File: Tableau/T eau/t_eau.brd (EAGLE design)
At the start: 70 x 60 mm, 24 parts

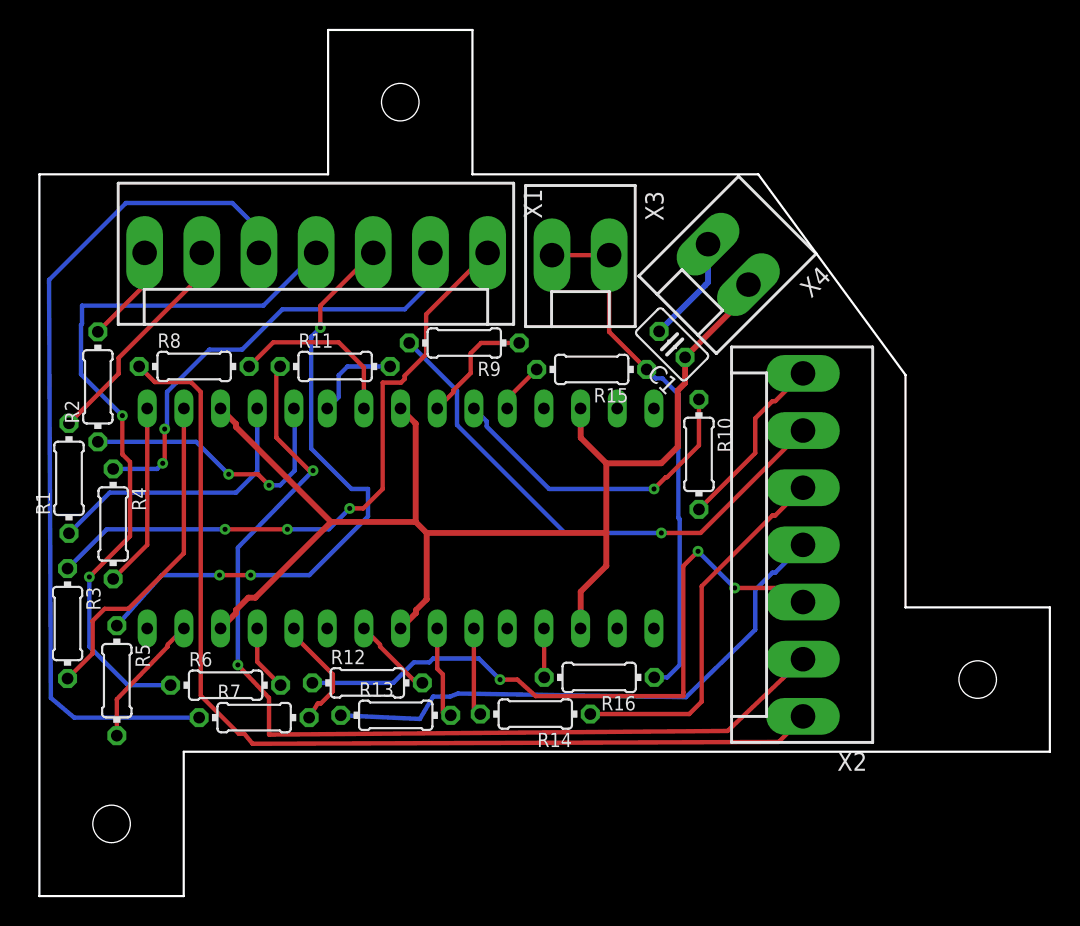
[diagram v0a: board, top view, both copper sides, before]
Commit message: no message
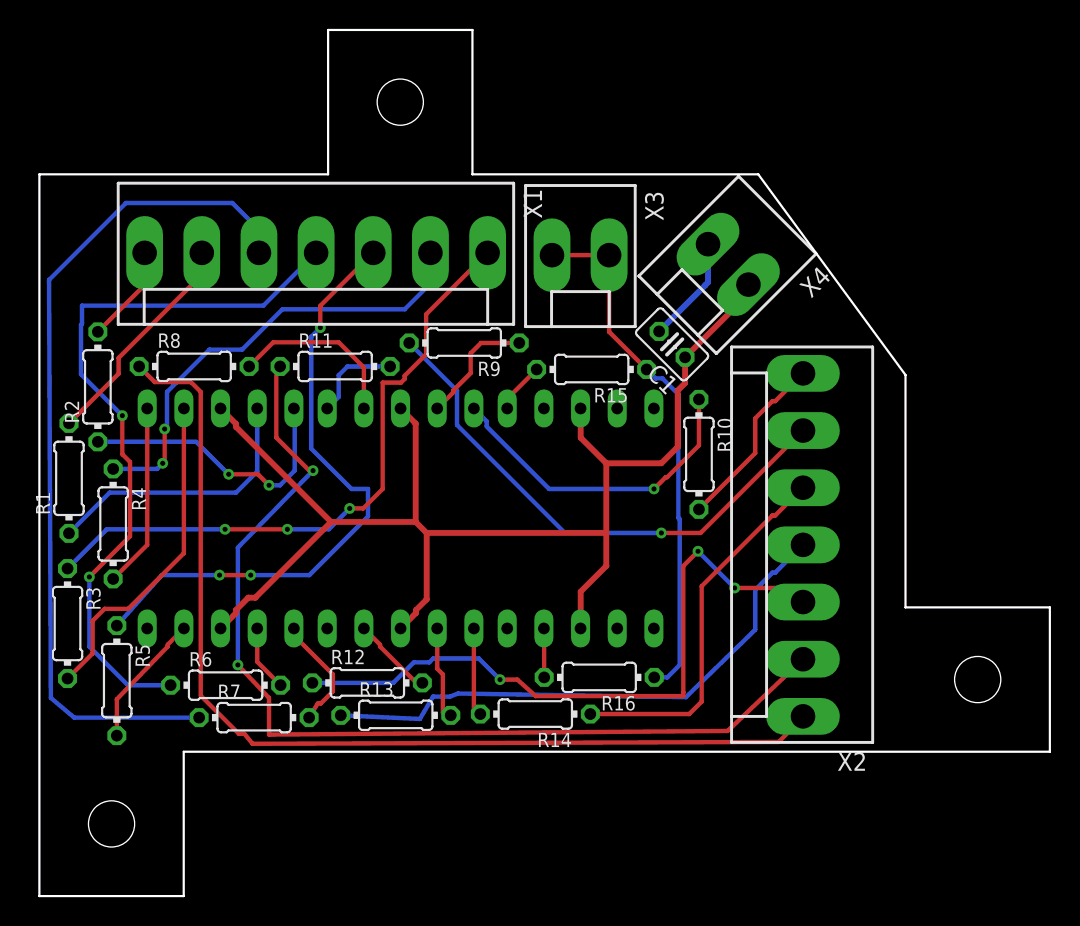
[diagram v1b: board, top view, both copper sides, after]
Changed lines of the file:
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@@
 <wire x1="20" y1="90" x2="20" y2="80" width="0.1524" layer="20"/>
 <wire x1="20" y1="80" x2="10" y2="80" width="0.1524" layer="20"/>
-<hole x="75" y="95" drill="2.6"/>
-<hole x="15" y="85" drill="2.6"/>
-<hole x="35" y="135" drill="2.6"/>
+<hole x="75" y="95" drill="3.2"/>
+<hole x="15" y="85" drill="3.2"/>
+<hole x="35" y="135" drill="3.2"/>
 </plain>
 <attributes>
